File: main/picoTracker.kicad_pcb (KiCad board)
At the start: 2 copper layers, 76 x 61 mm, 105 parts, among them IC1 XC6206P332MR, IC2 XC6206P332MR, IC3 BQ24232HRGTR, IC4 W25Q128JVS, IC5 PCM5102A, IC6 RP2040, IC7 TPA6139A2RGTR, IC8 H11L1, J1 5027740891, J2 USB_C_Receptacle_USB2.0, J3 Conn_01x02, J4 Conn_01x10, J5 Conn_01x18, J6 Headphones, J7 Conn_02x03_Odd_Even, J8 MIDI Out, J9 MIDI In, SW1 MS-22D28-G020, SW2 SW_SPST, Y1 12MHz 20pF ±10ppm

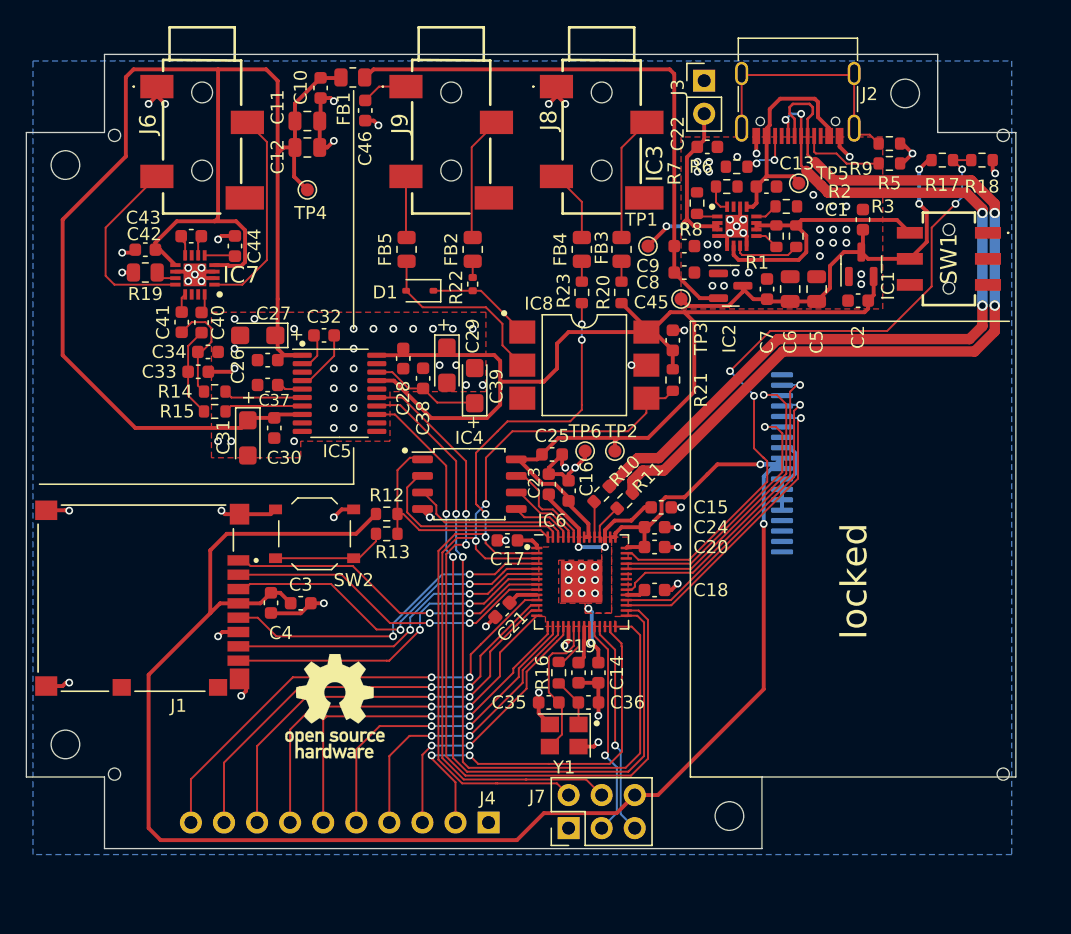
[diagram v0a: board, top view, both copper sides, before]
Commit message: picoTracker PCB v2.1 and picoTrackerKeypad PCB v2.0
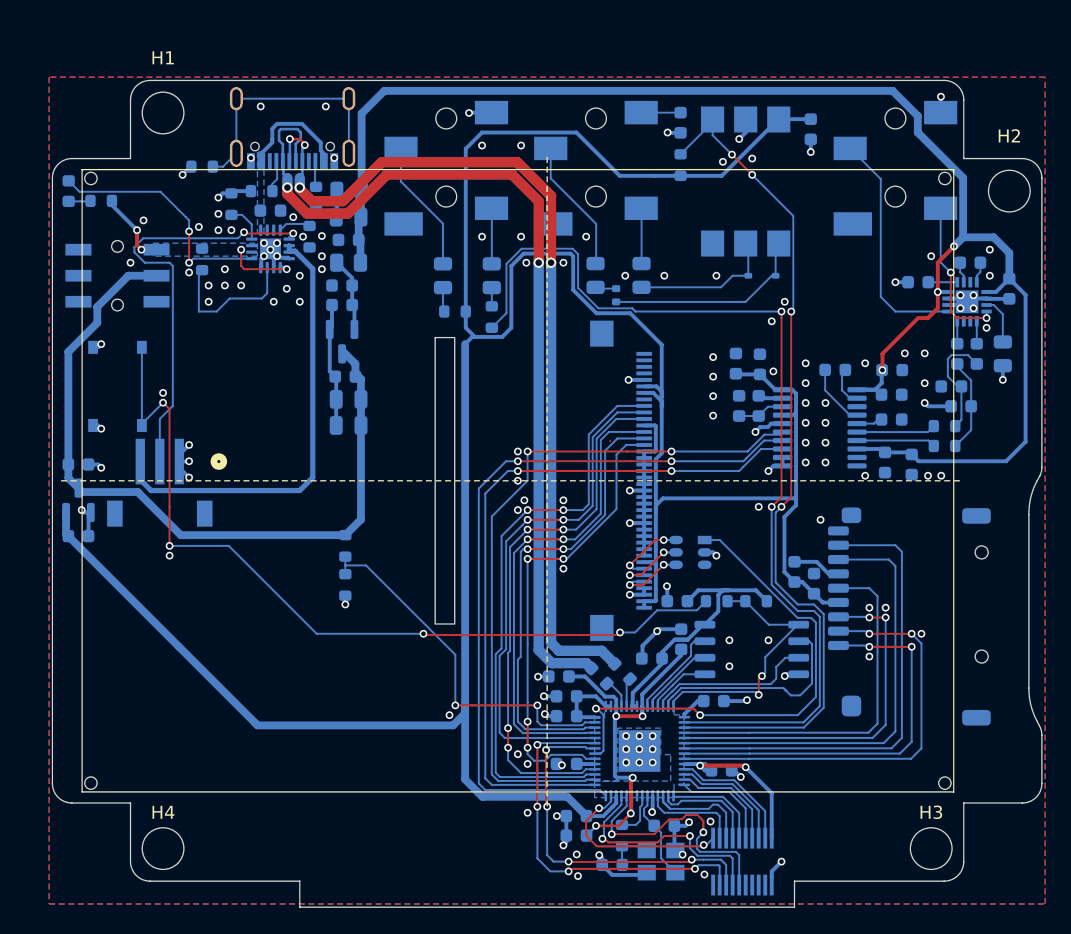
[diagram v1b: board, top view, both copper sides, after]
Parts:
- removed C39: 10uF, Capacitor_Tantalum_SMD:CP_EIA-3216-18_Kemet-A
- removed C41: 2.2uF, Capacitor_SMD:C_0603_1608Metric
- removed C42, C43, C44: 1uF, Capacitor_SMD:C_0603_1608Metric
- removed IC7: TPA6139A2RGTR, project:QFN50P300X300X100-17N-D
- removed J6: Headphones, project:PJ327C4A
- removed J7: Conn_02x03_Odd_Even, project:PinHeader_2x03_P2.54mm_Vertical
- removed R17, R18: 100k, Resistor_SMD:R_0603_1608Metric
- removed R19: 82k, Resistor_SMD:R_0805_2012Metric
- removed R7: 4.3k, Resistor_SMD:R_0603_1608Metric
- removed the REF** at (23.7, 50.1)
- removed TP1: VBAT, TestPoint:TestPoint_Pad_D1.0mm
- removed TP2: TestPoint, TestPoint:TestPoint_Pad_D1.0mm
- removed TP3: VCHR, TestPoint:TestPoint_Pad_D1.0mm
- removed TP4: 3.3VA, TestPoint:TestPoint_Pad_D1.0mm
- removed TP5: VBUS, TestPoint:TestPoint_Pad_D1.0mm
- removed TP6: GND, TestPoint:TestPoint_Pad_D1.0mm
- added C47: 1uF, Capacitor_SMD:C_0603_1608Metric, B.Cu at (72.5, 16.0)
- added C48: 2.2uF, Capacitor_SMD:C_0603_1608Metric, B.Cu at (73.0, 23.0)
- added C49: 1uF, Capacitor_SMD:C_0603_1608Metric, B.Cu at (75.5, 18.0)
- added C57: 1uF, Capacitor_SMD:C_0603_1608Metric, B.Cu at (18.8, 12.0)
- added D2: LED, LED_SMD:LED_0603_1608Metric, B.Cu at (3.25, 10.5)
- added J10: FPC-05FB-40PH20, project:FPC_40-flap, B.Cu at (40.0, 32.8)
- added R27: 1k, Resistor_SMD:R_0603_1608Metric, B.Cu at (15.8, 11.5)
- added R29: 560, Resistor_SMD:R_0603_1608Metric, B.Cu at (21.8, 14.0)
- added R4: 82k, Resistor_SMD:R_0805_2012Metric, B.Cu at (75.0, 23.0)
- added REF**: OSHW-Logo2_9.8x8mm_SilkScreen, Symbol:OSHW-Logo2_9.8x8mm_SilkScreen, B.Cu at (13.0, 50.3)
- added U1: AP2502KTR-G1, project:SOT23-6_DIO, B.Cu at (51.0, 38.2)
- added U2: BQ24074RGT, Package_DFN_QFN:VQFN-16-1EP_3x3mm_P0.5mm_EP1.6x1.6mm, B.Cu at (18.8, 14.9)
- C1, C10, C11, C12, C13, C14, C15, C16, C17, C18, C19, C2, C20, C21, C23, C24, C25, C26, C28, C3, C30, C32, C33, C34, C35, C36, C37, C38, C4, C45, C46, C5, C6, C7, C8, C9, D1, FB1, FB2, FB3, FB4, FB5, IC1, IC2, IC4, IC5, IC6, IC8, J2, J8, J9, R10, R11, R12, R13, R14, R15, R16, R20, R21, R22, R23, R5, R6, R9, SW1, SW2, Y1: moved to B.Cu
- C22: value 10uF -> 2.2uF; moved to B.Cu
- C27, C29, C31: footprint Capacitor_Tantalum_SMD:CP_EIA-3216-18_Kemet-A -> Capacitor_SMD:C_0603_1608Metric; moved to B.Cu
- C40: value 2.2uF -> 10uF; moved to B.Cu
- H1, H2, H3, H4: footprint MountingHole:MountingHole_2.2mm_M2 -> MountingHole:MountingHole_3.2mm_M3; moved to F.Cu
- IC3: value BQ24232HRGTR -> TPA6139A2RGTR; moved to B.Cu
- J1: value 5027740891 -> Conn_01x03; footprint project:MOLEX_5027740891 -> project:CONN_S3B-ZR-SM4A-TFLFSN_JST; moved to B.Cu
- J3: value Conn_01x02 -> Conn_02x10_Counter_Clockwise; footprint project:PinHeader_1x02_P2.54mm_Vertical -> Connector_Hirose:Hirose_DF12_DF12C3.0-20DS-0.5V_2x10_P0.50mm_Vertical; moved to B.Cu
- J4: value Conn_01x10 -> Micro_SD_Card; footprint project:PinHeader_1x10_P2.54mm_Vertical -> project:Xunpu_TF-115_microSD
- J5: value Conn_01x18 -> Headphones; footprint project:QD-TFT2803 -> project:PJ327C4A
- R1, R8: value 10k -> 1k; moved to B.Cu
- R2: value 3k -> 100k; moved to B.Cu
- R3: value 10k -> 100k; moved to B.Cu
- moved H2 72.5 mm to (75.5, 10.5), turned to 0 degrees
- moved H3 67.0 mm to (69.5, 61.0), turned to 0 degrees
- moved SW1 63.9 mm to (7.00, 17.0)
- moved C1 63.1 mm to (4.00, 31.5), turned to 0 degrees
- moved IC1 62.8 mm to (4.00, 34.2)
- moved C2 62.6 mm to (4.00, 37.0), turned to 0 degrees
- moved J3 60.1 mm to (55.0, 62.0), turned to 180 degrees
- moved C33 58.7 mm to (71.8, 27.0), turned to 180 degrees
- moved C34 57.2 mm to (71.0, 25.5), turned to 180 degrees
- moved H1 57.0 mm to (10.5, 4.50), turned to 0 degrees
- moved R14 56.1 mm to (70.5, 28.6), turned to 0 degrees
- moved R15 56.1 mm to (70.5, 30.1), turned to 0 degrees
- moved C40 53.2 mm to (66.5, 24.2), turned to 0 degrees
- moved R9 52.8 mm to (13.5, 8.62), turned to 180 degrees
- moved R1 51.9 mm to (5.75, 11.2), turned to 0 degrees
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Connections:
- net +1V1 renamed /+1.1V
- net /BCK renamed /DAC_I2S_BCK
- net /DIN renamed /DAC_I2S_DATA
- net /LRCK renamed /DAC_I2S_LRCK
- net Net-(IC2-VO) renamed /+3.3VApre
- C13 pad 1: VBUS -> Net-(IC3-VSS)
- C22 pad 1: /VBAT -> /LINE_OUT_R
- C22 pad 2: GND -> Net-(IC3--IN_L)
- C27 pad 1: +3.3VA -> +3V3
- C29 pad 1: +3V3 -> +3.3VA
- C31 pad 1: +3.3VA -> Net-(IC5-LDOO)
- C40 pad 1: /LINE_OUT_R -> +3.3VA
- C40 pad 2: Net-(IC7--IN_L) -> GND
- IC3 pad 1: Net-(IC3-TS) -> /OUT_HP_R
- IC3 pad 10: /VCHR1 -> GND
- IC3 pad 11: /VCHR1 -> Net-(IC3-GAIN)
- IC3 pad 12: Net-(IC3-ILIM) -> /OUT_HP_L
- IC3 pad 13: VBUS -> Net-(IC3--IN_R)
- IC3 pad 14: GND -> unconnected-(IC3-NC_2-Pad14)
- IC3 pad 16: Net-(IC3-ISET) -> Net-(IC3--IN_L)
- IC3 pad 2: /VBAT -> GND
- IC3 pad 3: /VBAT -> GND
- IC3 pad 4: GND -> +3.3VA
- IC3 pad 5: GND -> Net-(IC3-VSS)
- IC3 pad 6: /VCHR1 -> Net-(IC3-CN)
- IC3 pad 7: Net-(IC3-~{PGOOD}) -> unconnected-(IC3-NC_1-Pad7)
- IC3 pad 8: GND -> Net-(IC3-CP)
- IC3 pad 9: Net-(IC3-~{CHG}) -> +3.3VA
- IC6 pad 11: /SW_LEFT -> /INPUT_LEFT
- IC6 pad 12: /SW_DOWN -> /INPUT_DOWN
- IC6 pad 13: /SW_RIGHT -> /INPUT_RIGHT
- IC6 pad 14: /SW_UP -> /INPUT_UP
- IC6 pad 15: /SW_LT -> /INPUT_ALT
- IC6 pad 16: /SW_B -> /INPUT_EDIT
- IC6 pad 17: /SW_A -> /INPUT_ENTER
- IC6 pad 18: /SW_RT -> /INPUT_NAV
- IC6 pad 27: /SW_PLAY -> /INPUT_PLAY
- IC6 pad 35: /SCK -> /DISPLAY_PWM
- IC6 pad 36: /i2c0_SDA -> /DEBUG_TX
- IC6 pad 37: /i2c0_SCL -> /DEBUG_RX
- IC6 pad 40: /VOL -> /DISPLAY_MISO
- J1 pad 1: /SD_D2 -> GND
- J1 pad 2: /SD_D3 -> Net-(J1-Pin_2)
- J1 pad 3: /SD_CMD -> Net-(J1-Pin_3)
- J1 pad 4: +3V3 -> (no net)
- J1 pad 5: /SD_CLK -> (no net)
- J3 pad 1: GND -> +3V3
- J3 pad 2: /VBAT -> /INPUT_LEFT
- J4 pad 1: GND -> /SD_D2
- J4 pad 10: /SW_LEFT -> (no net)
- J4 pad 2: /SW_PLAY -> /SD_D3
- J4 pad 3: /SW_RT -> /SD_CMD
- J4 pad 4: /SW_A -> +3V3
- J4 pad 5: /SW_B -> /SD_CLK
- J4 pad 6: /SW_LT -> GND
- J4 pad 7: /SW_UP -> /SD_D0
- J4 pad 8: /SW_RIGHT -> /SD_D1
- J4 pad 9: /SW_DOWN -> GND
- J5 pad 2: /DISPLAY_RST -> /OUT_HP_L
- J5 pad 3: /DISPLAY_SCK -> /OUT_HP_R
- J5 pad 4: /DISPLAY_DC -> unconnected-(J5-Pad4)
- R1 pad 1: Net-(IC3-~{CHG}) -> Net-(D2-A)
- R2 pad 1: GND -> /VCHR2
- R2 pad 2: Net-(IC3-ILIM) -> /BAT
- R3 pad 1: Net-(IC3-~{PGOOD}) -> /BAT
- R3 pad 2: /VCHR1 -> GND
- R8 pad 1: GND -> /~{PGOOD}
- R8 pad 2: Net-(IC3-TS) -> /VCHR1
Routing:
- net /~{USB_BOOT}: track 8.42 -> 64.7 mm, vias 0 -> 4
- net /DISPLAY_PWM: track 0.00 -> 38.8 mm, vias 0 -> 2
- net /+3.3VApre: track 43.6 -> 5.86 mm
- net /SW_LEFT: track 36.6 -> 0.00 mm, vias 2 -> 0
- net /DISPLAY_MISO: track 0.00 -> 35.3 mm, vias 0 -> 2
- net /SW_DOWN: track 34.6 -> 0.00 mm, vias 2 -> 0
- net Net-(J1-Pin_3): track 0.00 -> 34.2 mm
- net /SW_RIGHT: track 32.8 -> 0.00 mm, vias 2 -> 0
- net Net-(J1-Pin_2): track 0.00 -> 31.5 mm, vias 0 -> 2
- net /SW_PLAY: track 31.2 -> 0.00 mm, vias 2 -> 0
- net /SW_UP: track 30.8 -> 0.00 mm, vias 2 -> 0
- net /DEBUG_RX: track 0.00 -> 28.8 mm, vias 0 -> 4
- net /SW_LT: track 28.6 -> 0.00 mm, vias 2 -> 0
- net /DEBUG_TX: track 0.00 -> 27.3 mm, vias 0 -> 4
- net /VCHR2: track 32.6 -> 58.0 mm, vias 2 -> 0
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- added copper zone on B.Cu, net +3V3
- added copper zone on B.Cu, net /VCHR1
- added copper zone on B.Cu, net VBUS
- removed copper zone on F.Cu, net +3V3
- removed copper zone on F.Cu, net /+1.1V
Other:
- board size 76 x 61 mm -> 76 x 63.5 mm
- board text added: "Battery LIP1708"
- board text added: "xiphonics picoTracker v2.1"
- board text removed: "A"
- board text removed: "B"
- board text removed: "D"
- board text removed: "L"
- board text removed: "LT"
- board text removed: "P"
- board text removed: "R"
- board text removed: "RT"
- board text removed: "U"
- board text removed: "gnd"
- board text removed: "https://github.com/democloid/picoTracker"
- board text removed: "io clk"
- board text removed: "locked"
- board text removed: "picoTrackerPortable v1.1"
- board text removed: "rx tx"
- board text removed: "swd"
- board text removed: "vcc"
